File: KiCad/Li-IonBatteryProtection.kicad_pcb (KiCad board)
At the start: 2 copper layers, 1 part, among them Q1 IRF540N

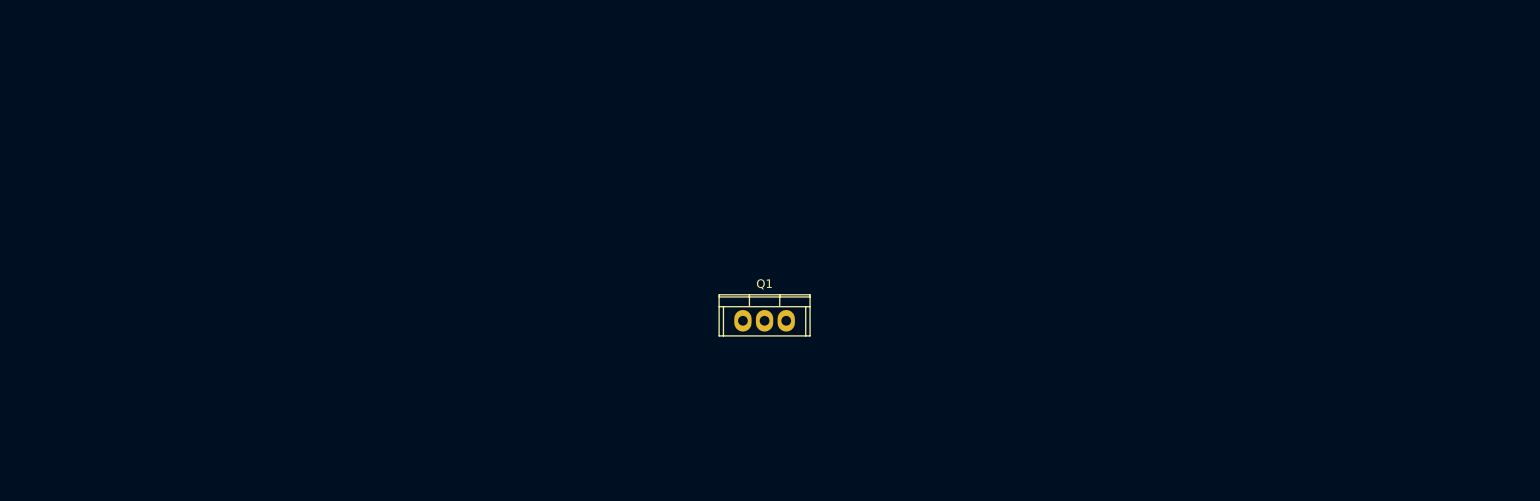
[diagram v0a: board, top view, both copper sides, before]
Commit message: Net wiring on PCB is done.
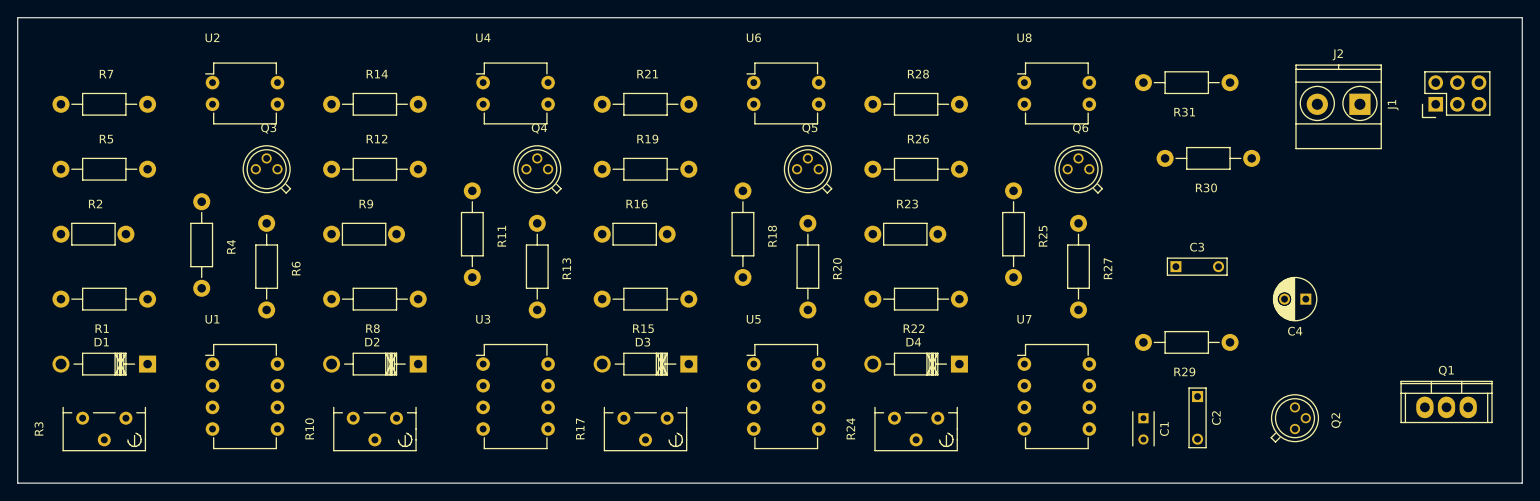
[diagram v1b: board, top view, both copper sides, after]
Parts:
- added C1: 0.1uf, Capacitors_ThroughHole:C_Rect_L4_W2.5_P2.5, F.Cu at (184.2, 119.4)
- added C2: 0.22uf, Capacitors_ThroughHole:C_Rect_L7_W2_P5, F.Cu at (190.5, 116.8)
- added C3: 0.001uf, Capacitors_ThroughHole:C_Rect_L7_W2_P5, F.Cu at (188.0, 101.6)
- added C4: 47uf, Capacitors_ThroughHole:C_Radial_D5_L11_P2.5, F.Cu at (203.2, 105.4)
- added D1: 1N4728, Diodes_ThroughHole:Diode_DO-41_SOD81_Horizontal_RM10, F.Cu at (67.3, 113.0)
- added D2: 1N4728, Diodes_ThroughHole:Diode_DO-41_SOD81_Horizontal_RM10, F.Cu at (99.1, 113.0)
- added D3: 1N4728, Diodes_ThroughHole:Diode_DO-41_SOD81_Horizontal_RM10, F.Cu at (130.8, 113.0)
- added D4: 1N4728, Diodes_ThroughHole:Diode_DO-41_SOD81_Horizontal_RM10, F.Cu at (162.6, 113.0)
- added J1: CONN_02X03, Pin_Headers:Pin_Header_Straight_2x03, F.Cu at (218.4, 82.5)
- added J2: CONN_01X02, Terminal_Blocks:TerminalBlock_Pheonix_MKDS1.5-2pol, F.Cu at (209.6, 82.5)
- added Q2: 2N2222A, TO_SOT_Packages_THT:TO-18_3Pin, F.Cu at (201.9, 119.4)
- added Q3: 2N2222A, TO_SOT_Packages_THT:TO-18_3Pin, F.Cu at (81.3, 90.2)
- added Q4: 2N2222A, TO_SOT_Packages_THT:TO-18_3Pin, F.Cu at (113.0, 90.2)
- added Q5: 2N2222A, TO_SOT_Packages_THT:TO-18_3Pin, F.Cu at (144.8, 90.2)
- added Q6: 2N2222A, TO_SOT_Packages_THT:TO-18_3Pin, F.Cu at (176.5, 90.2)
- added R1: 10k, Resistors_ThroughHole:Resistor_Horizontal_RM10mm, F.Cu at (67.3, 105.4)
- added R10: 1Meg, Potentiometers:Potentiometer_Bourns_3296Y_3-8Zoll_Angular_ScrewUp, F.Cu at (96.5, 119.4)
- added R11: 47k, Resistors_ThroughHole:Resistor_Horizontal_RM10mm, F.Cu at (105.4, 92.7)
- added R12: 100k, Resistors_ThroughHole:Resistor_Horizontal_RM10mm, F.Cu at (88.9, 90.2)
- added R13: 100, Resistors_ThroughHole:Resistor_Horizontal_RM10mm, F.Cu at (113.0, 96.5)
- added R14: 120, Resistors_ThroughHole:Resistor_Horizontal_RM10mm, F.Cu at (88.9, 82.5)
- added R15: 10k, Resistors_ThroughHole:Resistor_Horizontal_RM10mm, F.Cu at (130.8, 105.4)
- added R16: 1k, Resistors_ThroughHole:Resistor_Horizontal_RM7mm, F.Cu at (120.7, 97.8)
- added R17: 1Meg, Potentiometers:Potentiometer_Bourns_3296Y_3-8Zoll_Angular_ScrewUp, F.Cu at (128.3, 119.4)
- added R18: 47k, Resistors_ThroughHole:Resistor_Horizontal_RM10mm, F.Cu at (137.2, 92.7)
- added R19: 100k, Resistors_ThroughHole:Resistor_Horizontal_RM10mm, F.Cu at (120.7, 90.2)
- added R2: 1k, Resistors_ThroughHole:Resistor_Horizontal_RM7mm, F.Cu at (57.1, 97.8)
- added R20: 100, Resistors_ThroughHole:Resistor_Horizontal_RM10mm, F.Cu at (144.8, 96.5)
- added R21: 120, Resistors_ThroughHole:Resistor_Horizontal_RM10mm, F.Cu at (120.7, 82.5)
- added R22: 10k, Resistors_ThroughHole:Resistor_Horizontal_RM10mm, F.Cu at (162.6, 105.4)
- added R23: 1k, Resistors_ThroughHole:Resistor_Horizontal_RM7mm, F.Cu at (152.4, 97.8)
- added R24: 1Meg, Potentiometers:Potentiometer_Bourns_3296Y_3-8Zoll_Angular_ScrewUp, F.Cu at (160.0, 119.4)
- added R25: 47k, Resistors_ThroughHole:Resistor_Horizontal_RM10mm, F.Cu at (168.9, 92.7)
- added R26: 100k, Resistors_ThroughHole:Resistor_Horizontal_RM10mm, F.Cu at (152.4, 90.2)
- added R27: 100, Resistors_ThroughHole:Resistor_Horizontal_RM10mm, F.Cu at (176.5, 96.5)
- added R28: 120, Resistors_ThroughHole:Resistor_Horizontal_RM10mm, F.Cu at (152.4, 82.5)
- added R29: 5.1k, Resistors_ThroughHole:Resistor_Horizontal_RM10mm, F.Cu at (194.3, 110.5)
- added R3: 1Meg, Potentiometers:Potentiometer_Bourns_3296Y_3-8Zoll_Angular_ScrewUp, F.Cu at (64.8, 119.4)
- added R30: 3.3k, Resistors_ThroughHole:Resistor_Horizontal_RM10mm, F.Cu at (196.8, 88.9)
- added R31: 20k, Resistors_ThroughHole:Resistor_Horizontal_RM10mm, F.Cu at (194.3, 80.0)
- added R4: 47k, Resistors_ThroughHole:Resistor_Horizontal_RM10mm, F.Cu at (73.7, 94.0)
- added R5: 100k, Resistors_ThroughHole:Resistor_Horizontal_RM10mm, F.Cu at (57.1, 90.2)
- added R6: 100, Resistors_ThroughHole:Resistor_Horizontal_RM10mm, F.Cu at (81.3, 96.5)
- added R7: 120, Resistors_ThroughHole:Resistor_Horizontal_RM10mm, F.Cu at (57.1, 82.5)
- added R8: 10k, Resistors_ThroughHole:Resistor_Horizontal_RM10mm, F.Cu at (99.1, 105.4)
- added R9: 1k, Resistors_ThroughHole:Resistor_Horizontal_RM7mm, F.Cu at (88.9, 97.8)
- added U1: LM311N, Housings_DIP:DIP-8_W7.62mm, F.Cu at (74.9, 113.0)
- added U2: PC817, Housings_DIP:DIP-4_W7.62mm, F.Cu at (74.9, 80.0)
- added U3: LM311N, Housings_DIP:DIP-8_W7.62mm, F.Cu at (106.7, 113.0)
- added U4: PC817, Housings_DIP:DIP-4_W7.62mm, F.Cu at (106.7, 80.0)
- added U5: LM311N, Housings_DIP:DIP-8_W7.62mm, F.Cu at (138.4, 113.0)
- added U6: PC817, Housings_DIP:DIP-4_W7.62mm, F.Cu at (138.4, 80.0)
- added U7: LM311N, Housings_DIP:DIP-8_W7.62mm, F.Cu at (170.2, 113.0)
- added U8: PC817, Housings_DIP:DIP-4_W7.62mm, F.Cu at (170.2, 80.0)
- moved Q1 80.7 mm to (219.7, 118.1)
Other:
- board outline added: 176.5 x 54.6 mm
